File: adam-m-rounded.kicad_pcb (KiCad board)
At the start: 2 copper layers, 114.5 x 95.3 mm, 21 parts, among them J1 AudioJack4dpb, SW1 SW_Push, SW10 SW_Push, SW11 SW_Push, SW12 SW_Push, SW13 SW_Push, SW14 SW_Push, SW15 SW_Push, SW16 SW_Push, SW17 SW_Push, SW2 SW_Push, SW3 SW_Push, SW4 SW_Push, SW5 SW_Push, SW6 SW_Push, SW7 SW_Push, SW8 SW_Push, SW9 SW_Push, U1 ProMicro-kbd

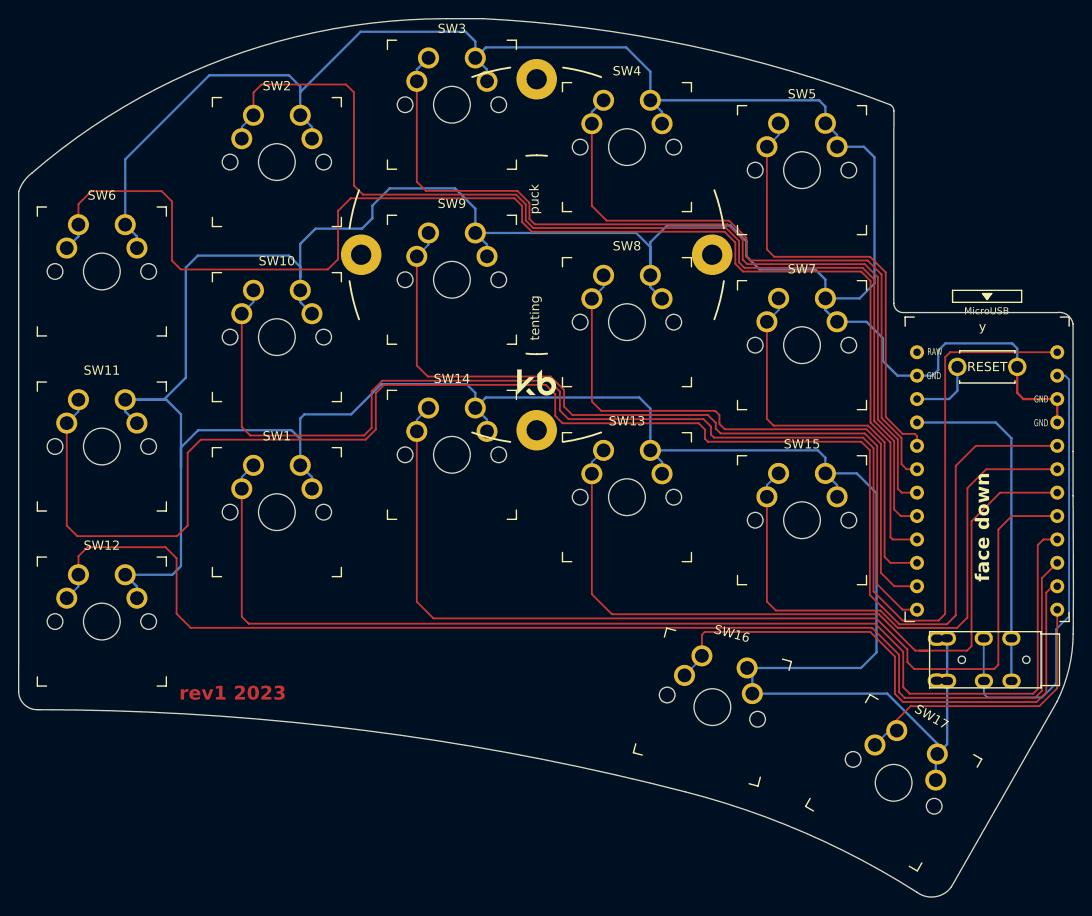
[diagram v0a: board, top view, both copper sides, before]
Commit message: add gerbers
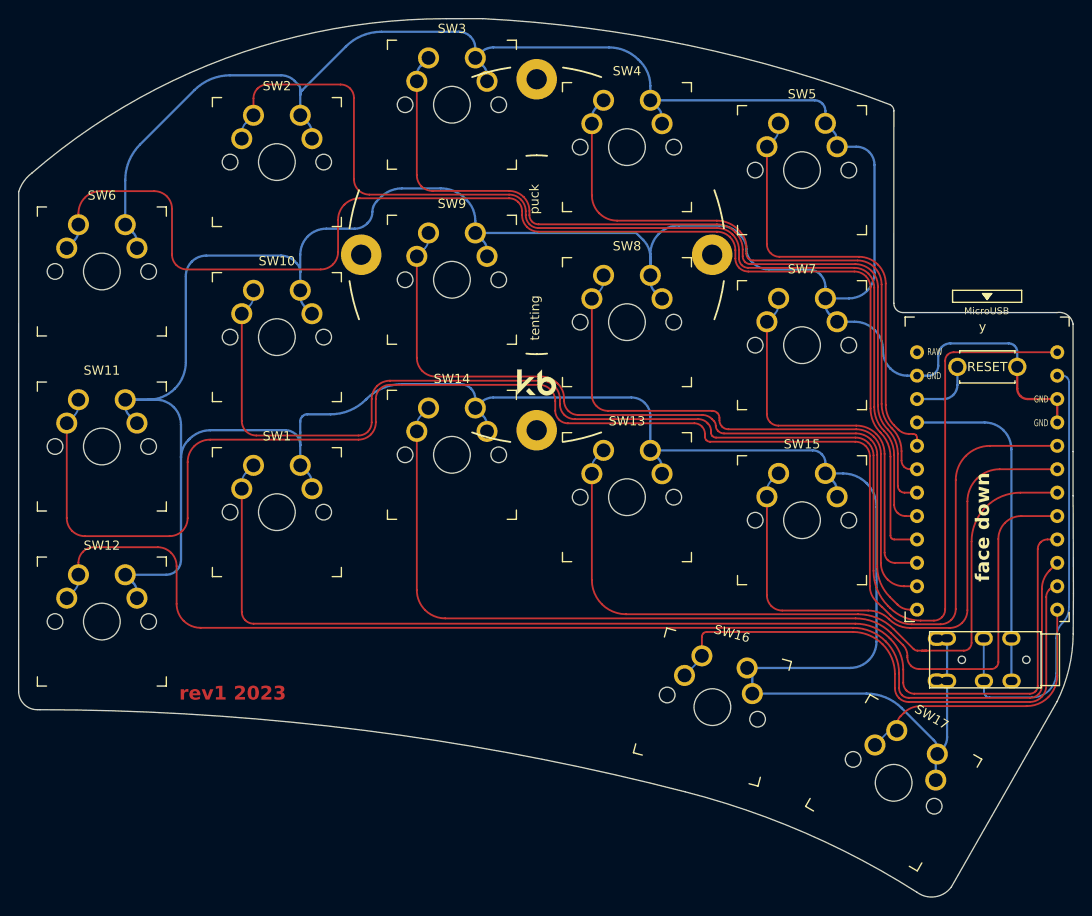
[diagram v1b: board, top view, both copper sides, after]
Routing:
- net gnd: track 526.2 -> 486.7 mm
- net Switch11: track 175.4 -> 172.3 mm
- net Switch6: track 143.2 -> 140.3 mm
- net Switch10: track 159.0 -> 156.5 mm
- net Switch2: track 119.0 -> 116.5 mm
- net Switch13: track 85.0 -> 82.8 mm
- net Switch3: track 96.7 -> 94.5 mm
- net Switch15: track 137.6 -> 135.5 mm
- net Switch9: track 90.4 -> 88.4 mm
- net Switch4: track 71.1 -> 69.1 mm
- net Switch14: track 110.4 -> 108.6 mm
- net Switch12: track 62.5 -> 60.8 mm
- net Switch1: track 127.3 -> 125.7 mm
- net Switch8: track 66.6 -> 65.1 mm
- net Switch5: track 49.1 -> 47.8 mm
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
